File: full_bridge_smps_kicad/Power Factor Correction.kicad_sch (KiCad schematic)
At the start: 44 parts, among them Q2 MMBT2904, Q5 IPA60R280C6, Q6 IPA60R280C6, Q6 SI2309, Q7 IPW60R041C6, T1 PA1005.100NL, T2 PA1005.100NL, U4 TL431ACDBZR, U5 UCC27324D, U6 UCC27324D

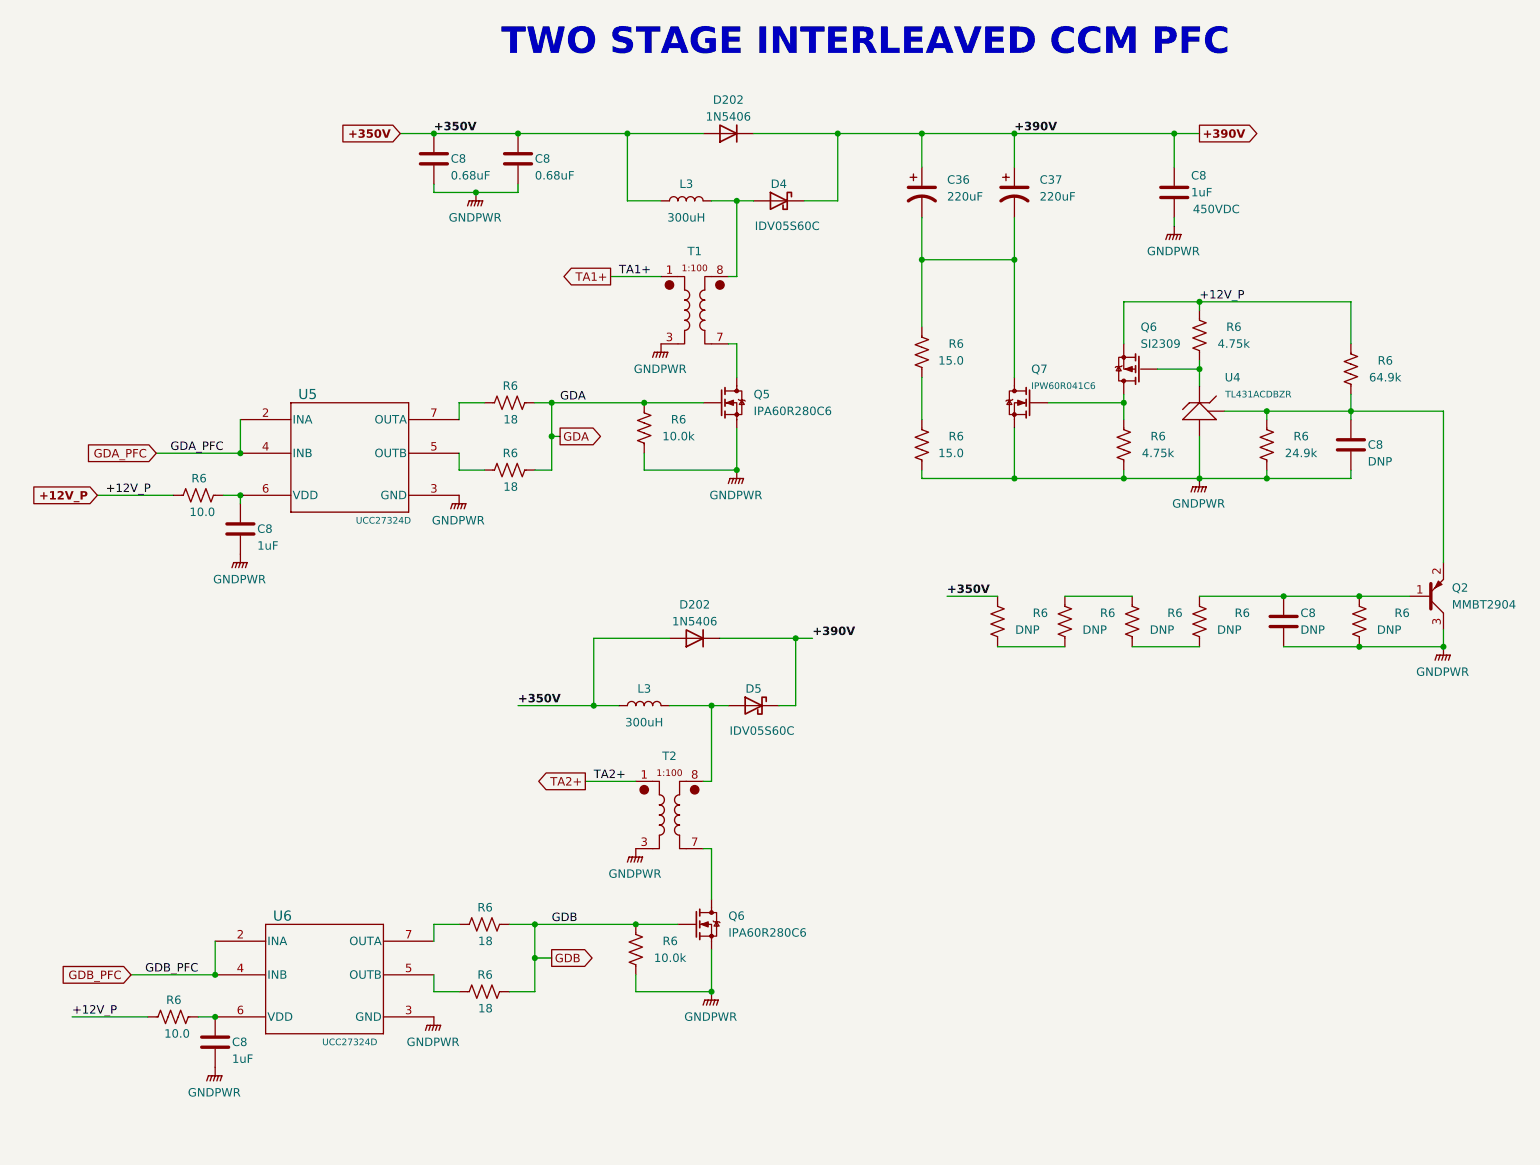
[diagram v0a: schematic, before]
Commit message: A bit of refactoring, saving work for the day
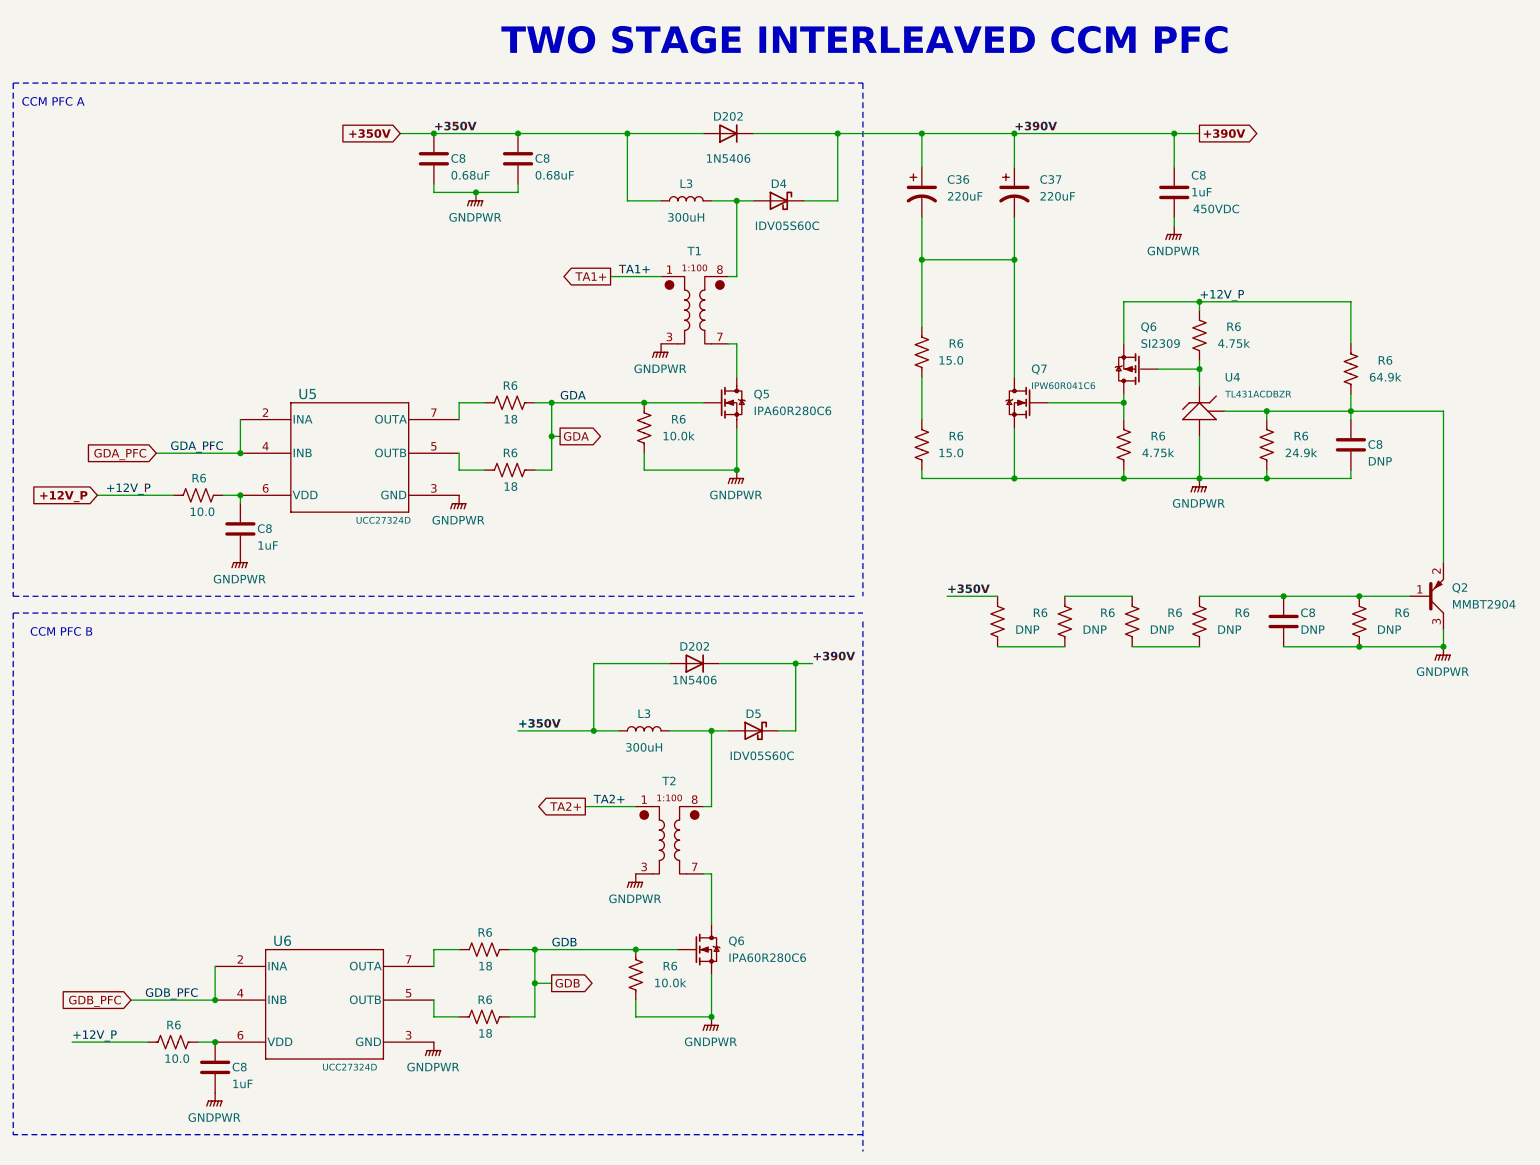
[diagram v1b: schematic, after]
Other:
- note added: "CCM PFC A"
- note added: "CCM PFC B"
- moved on the sheet: C8, D202, D5, L3, Q6, R6, T2, U6
